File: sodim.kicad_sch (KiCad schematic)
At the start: 1 part, among them J1 ddr4-sodimm-edge-connector

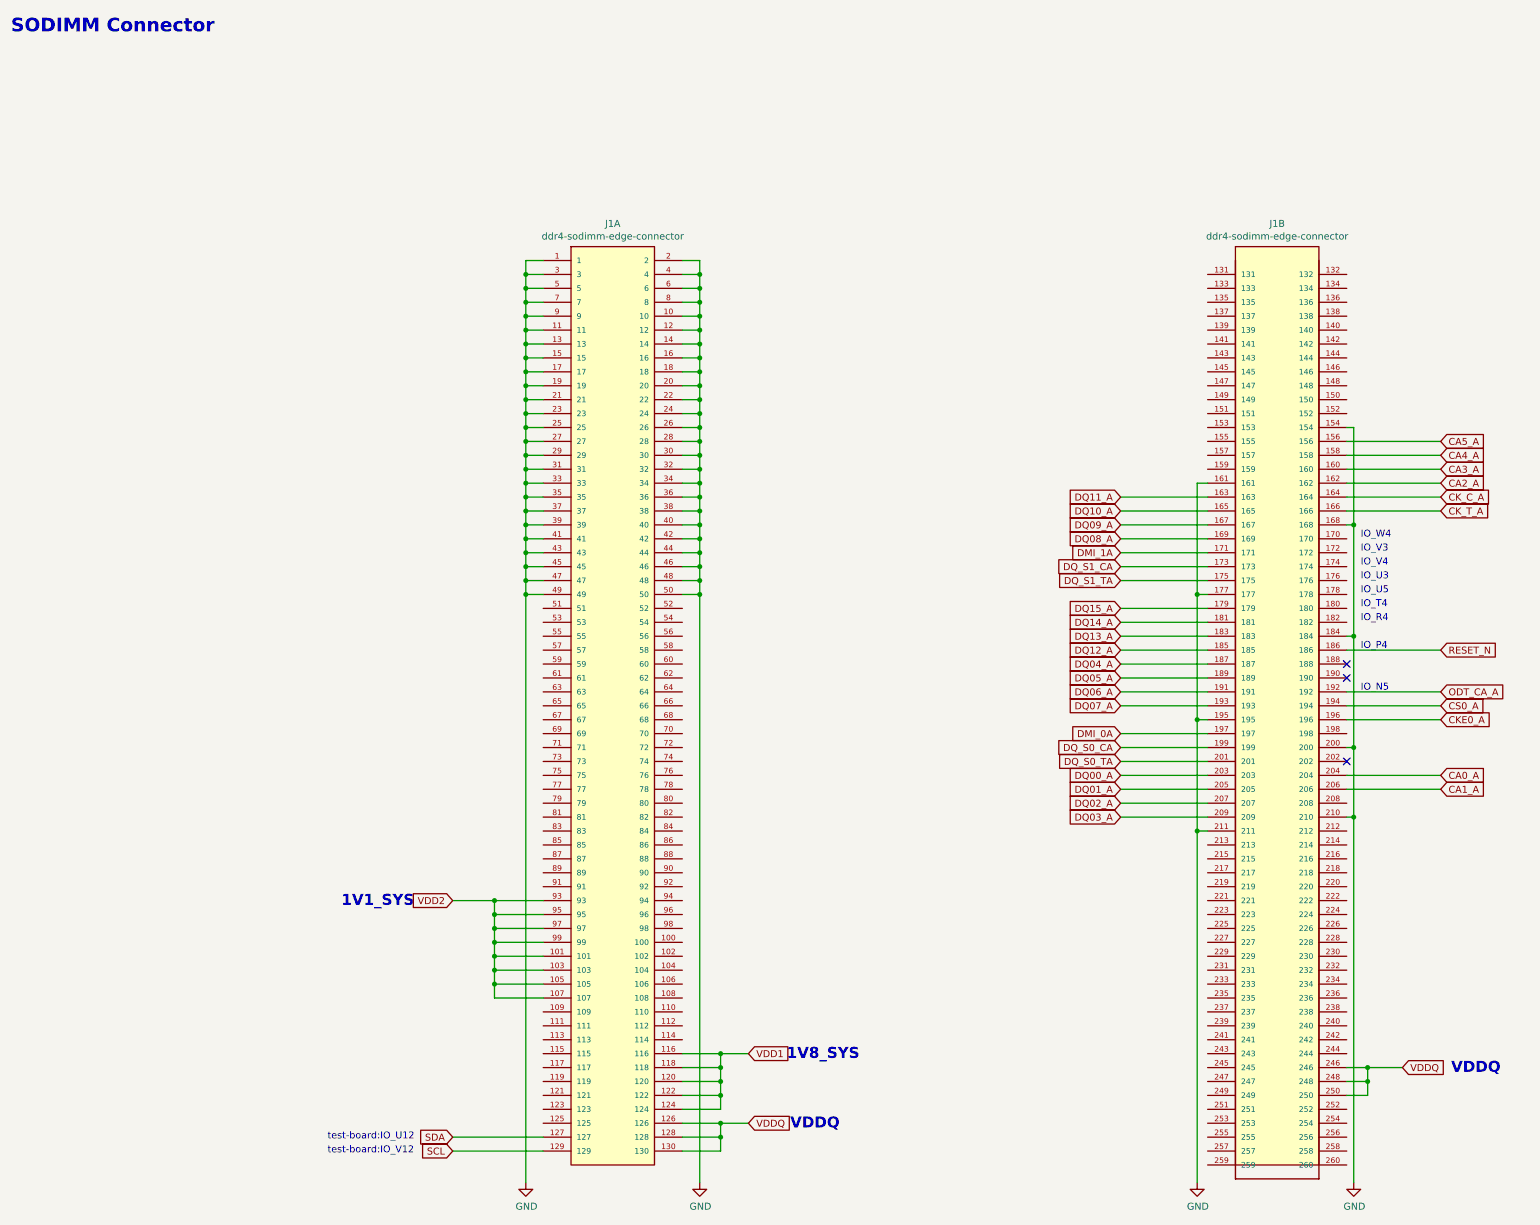
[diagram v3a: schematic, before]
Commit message: Fix missing global links (wip), designators fixed
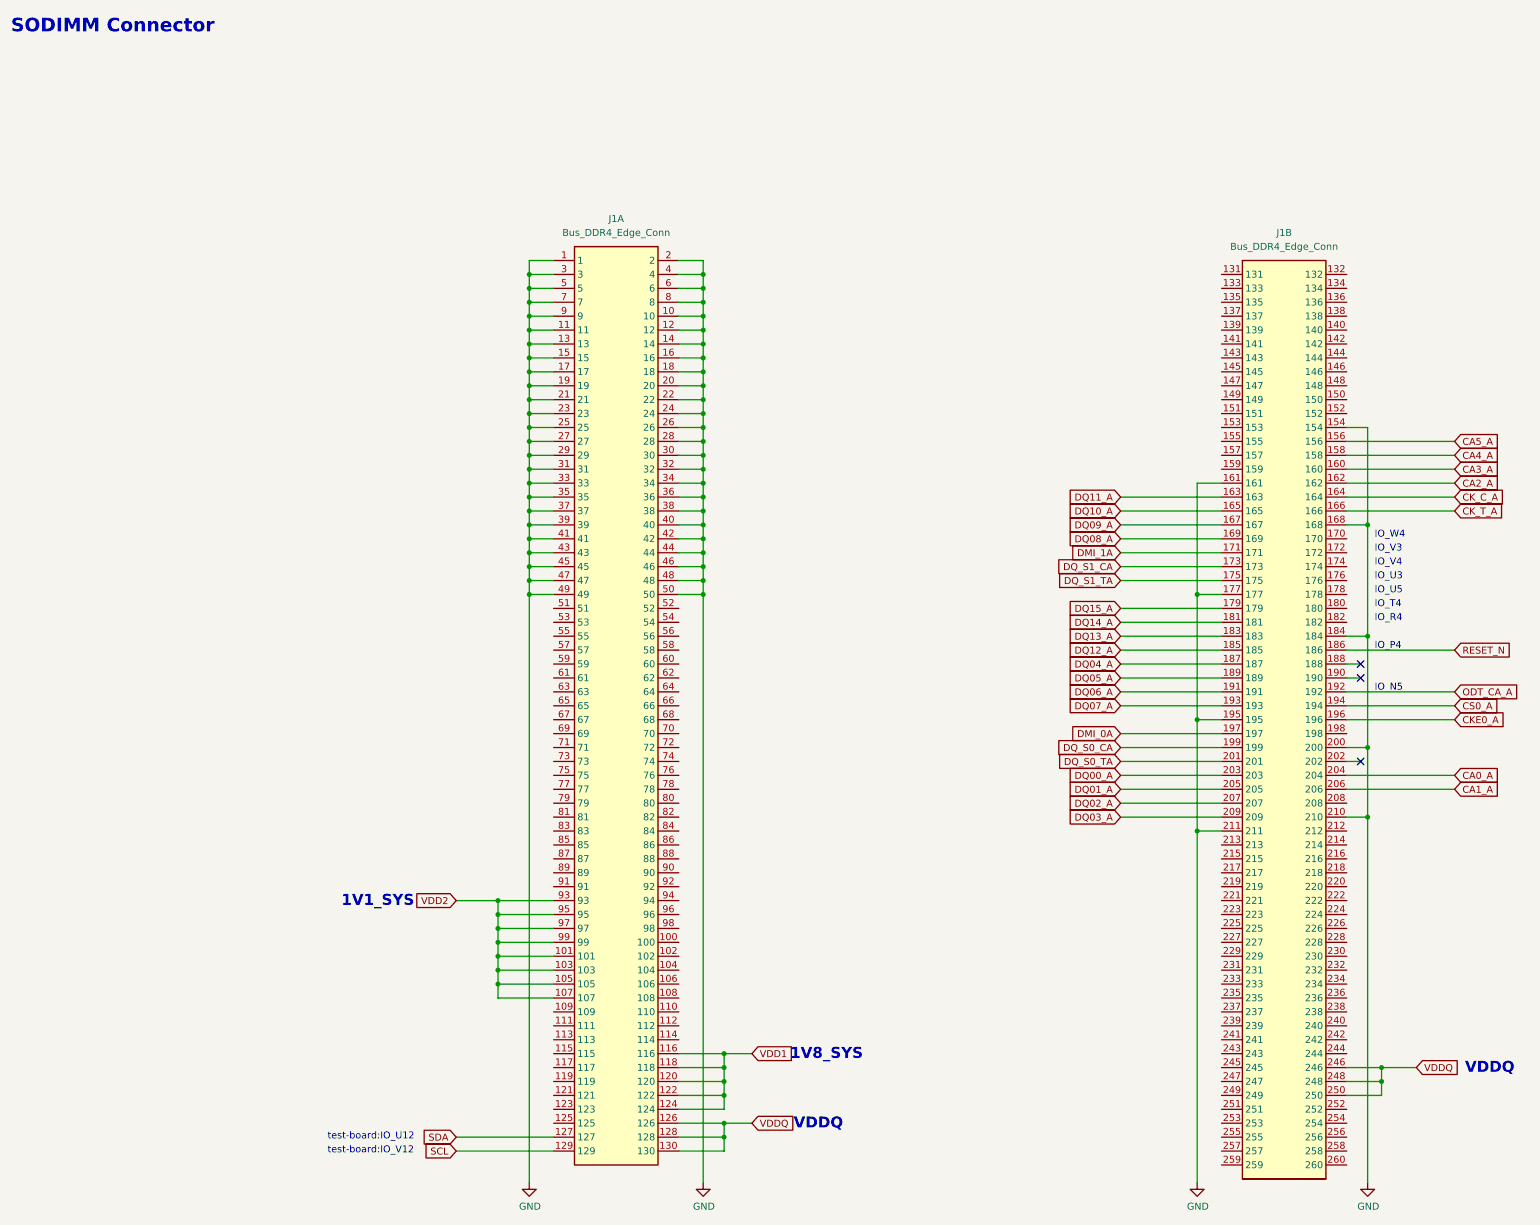
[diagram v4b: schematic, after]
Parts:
- removed J1: ddr4-sodimm-edge-connector, lpddr4-testbed-footprints:SODIMM_DDR4_EDGE, symbol lpddr4-testbed:ddr4-sodimm-edge-connector
- added J1: Bus_DDR4_Edge_Conn, antmicro-footprints:Bus_DDR4_Conn_Edge, symbol antmicroMemoryConnectorsPCCardSockets:Bus_DDR4_Edge_Conn
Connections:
- net CA0_A: now also J1.204
- net CA1_A: now also J1.206
- net CA2_A: now also J1.162
- net CA3_A: now also J1.160
- net CA4_A: now also J1.158
- net CA5_A: now also J1.156
- net CKE0_A: now also J1.196
- net CK_C_A: now also J1.164
- net CK_T_A: now also J1.166
- net CS0_A: now also J1.194
- net DMI_0A: now also J1.197
- net DMI_1A: now also J1.171
- net DQ00_A: now also J1.203
- net DQ01_A: now also J1.205
- net DQ02_A: now also J1.207
- net DQ03_A: now also J1.209
- net DQ04_A: now also J1.187
- net DQ05_A: now also J1.189
- net DQ06_A: now also J1.191
- net DQ07_A: now also J1.193
- net DQ08_A: now also J1.169
- net DQ09_A: now also J1.167
- net DQ10_A: now also J1.165
- net DQ11_A: now also J1.163
- net DQ12_A: now also J1.185
- net DQ13_A: now also J1.183
- net DQ14_A: now also J1.181
- net DQ15_A: now also J1.179
- net DQ_S0_CA: now also J1.199
- net DQ_S0_TA: now also J1.201
- net DQ_S1_CA: now also J1.173
- net DQ_S1_TA: now also J1.175
- net GND: now also J1.1, J1.10, J1.11, J1.12, J1.13, J1.14, J1.15, J1.154, J1.16, J1.161, J1.168, J1.17, J1.177, J1.18, J1.184, J1.19, J1.195, J1.2, J1.20, J1.200, J1.21, J1.210, J1.211, J1.22, J1.23, J1.24, J1.25, J1.26, J1.27, J1.28, J1.29, J1.3, J1.30, J1.31, J1.32, J1.33, J1.34, J1.35, J1.36, J1.37, J1.38, J1.39, J1.4, J1.40, J1.41, J1.42, J1.43, J1.44, J1.45, J1.46, J1.47, J1.48, J1.49, J1.5, J1.50, J1.6, J1.7, J1.8, J1.9
- net ODT_CA_A: now also J1.192
- net RESET_N: now also J1.186
- net SCL: now also J1.129
- net SDA: now also J1.127
- net VDD1: now also J1.116, J1.118, J1.120, J1.122, J1.124
- net VDD2: now also J1.101, J1.103, J1.105, J1.107, J1.93, J1.95, J1.97, J1.99
- net VDDQ: now also J1.126, J1.128, J1.130, J1.246, J1.248, J1.250
